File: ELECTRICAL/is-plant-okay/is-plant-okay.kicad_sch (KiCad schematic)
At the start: 0 parts

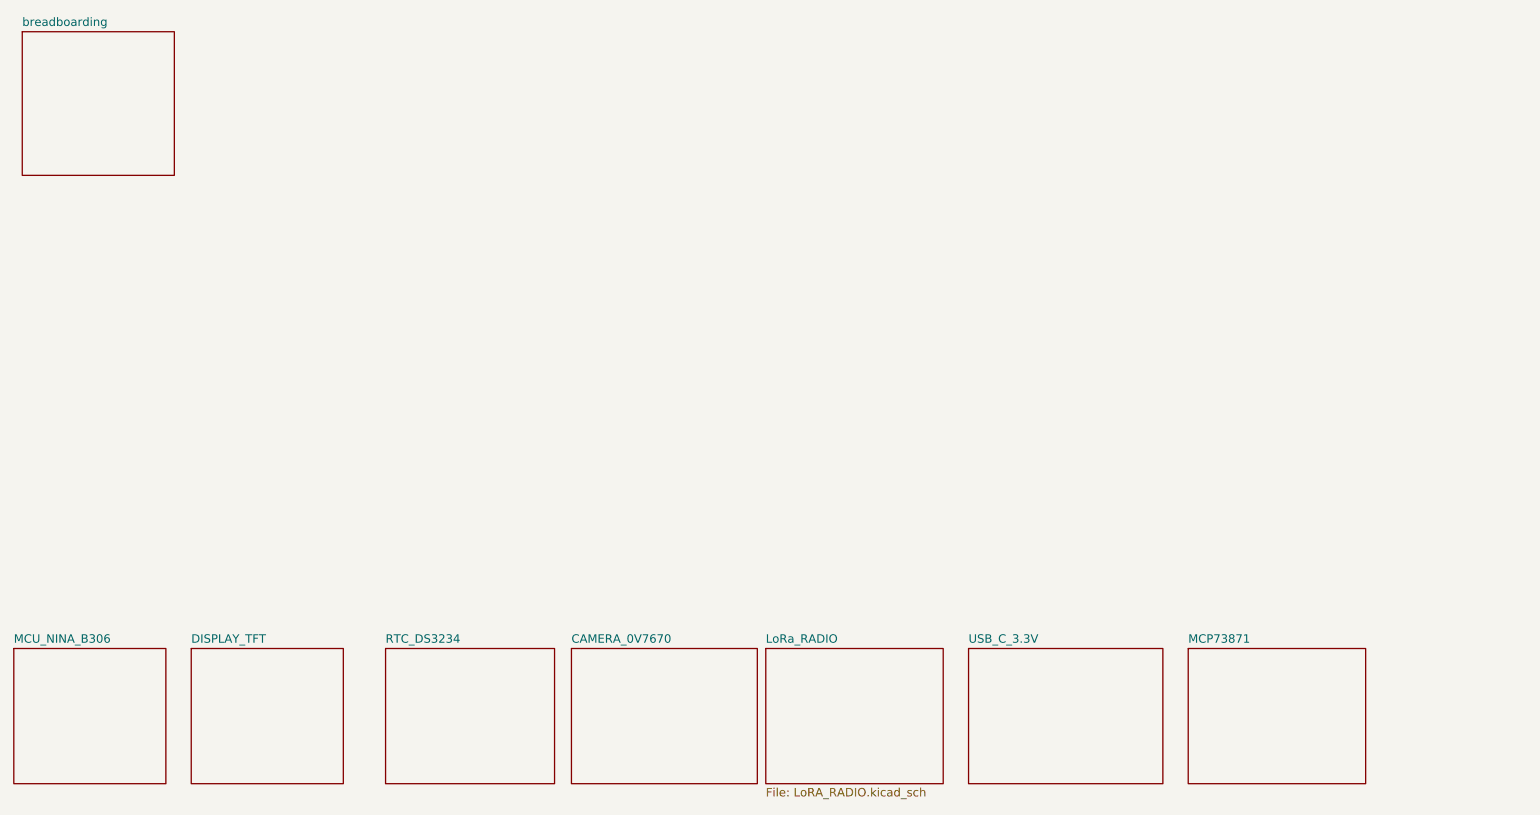
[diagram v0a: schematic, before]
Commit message: feat: finished schematics
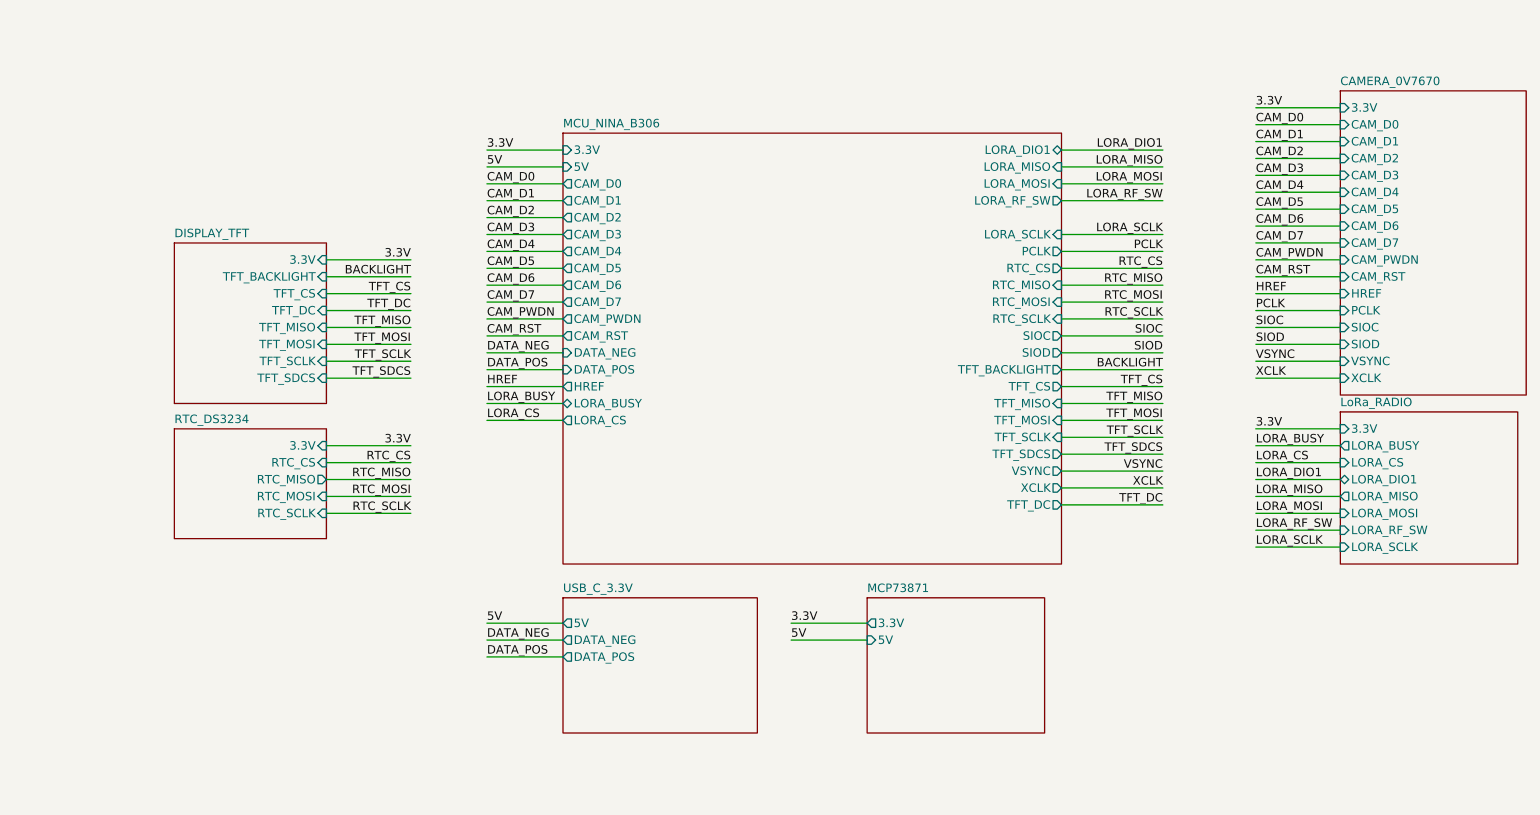
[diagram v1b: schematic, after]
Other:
- removed sheet breadboarding
- sheet CAMERA_0V7670 ports: added 3.3V, CAM_D0, CAM_D1, CAM_D2, CAM_D3, CAM_D4, CAM_D5, CAM_D6, CAM_D7, CAM_PWDN, CAM_RST, HREF, PCLK, SIOC, SIOD, VSYNC, XCLK; removed none
- sheet DISPLAY_TFT ports: added 3.3V, TFT_BACKLIGHT, TFT_CS, TFT_DC, TFT_MISO, TFT_MOSI, TFT_SCLK, TFT_SDCS; removed none
- sheet LoRa_RADIO ports: added 3.3V, LORA_BUSY, LORA_CS, LORA_DIO1, LORA_MISO, LORA_MOSI, LORA_RF_SW, LORA_SCLK; removed none
- sheet MCP73871 ports: added 3.3V, 5V; removed none
- sheet MCU_NINA_B306 ports: added 3.3V, 5V, CAM_D0, CAM_D1, CAM_D2, CAM_D3, CAM_D4, CAM_D5, CAM_D6, CAM_D7, CAM_PWDN, CAM_RST, DATA_NEG, DATA_POS, HREF, LORA_BUSY, LORA_CS, LORA_DIO1, LORA_MISO, LORA_MOSI, LORA_RF_SW, LORA_SCLK, PCLK, RTC_CS, RTC_MISO, RTC_MOSI, RTC_SCLK, SIOC, SIOD, TFT_BACKLIGHT, TFT_CS, TFT_DC, TFT_MISO, TFT_MOSI, TFT_SCLK, TFT_SDCS, VSYNC, XCLK; removed none
- sheet RTC_DS3234 ports: added 3.3V, RTC_CS, RTC_MISO, RTC_MOSI, RTC_SCLK; removed none
- sheet USB_C_3.3V ports: added 5V, DATA_NEG, DATA_POS; removed none
